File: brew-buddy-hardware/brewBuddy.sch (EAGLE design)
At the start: 3 parts

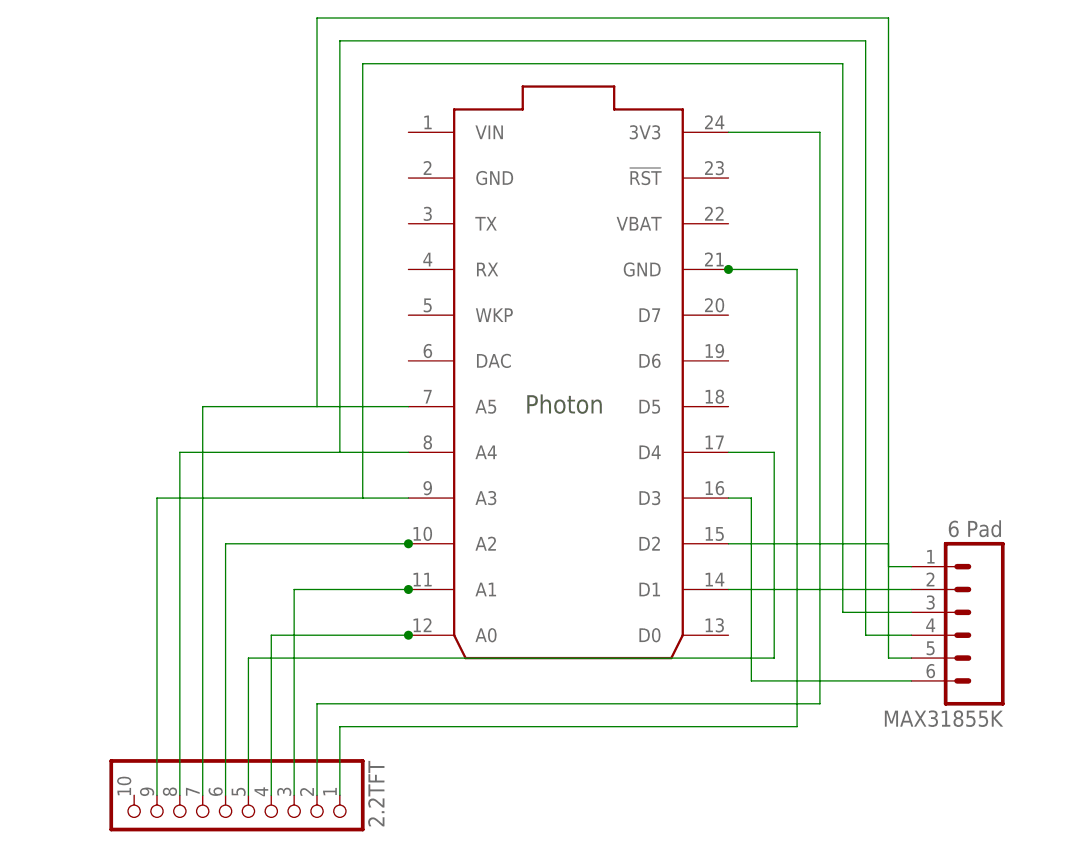
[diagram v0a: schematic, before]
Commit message: updated schematic and board for Argon
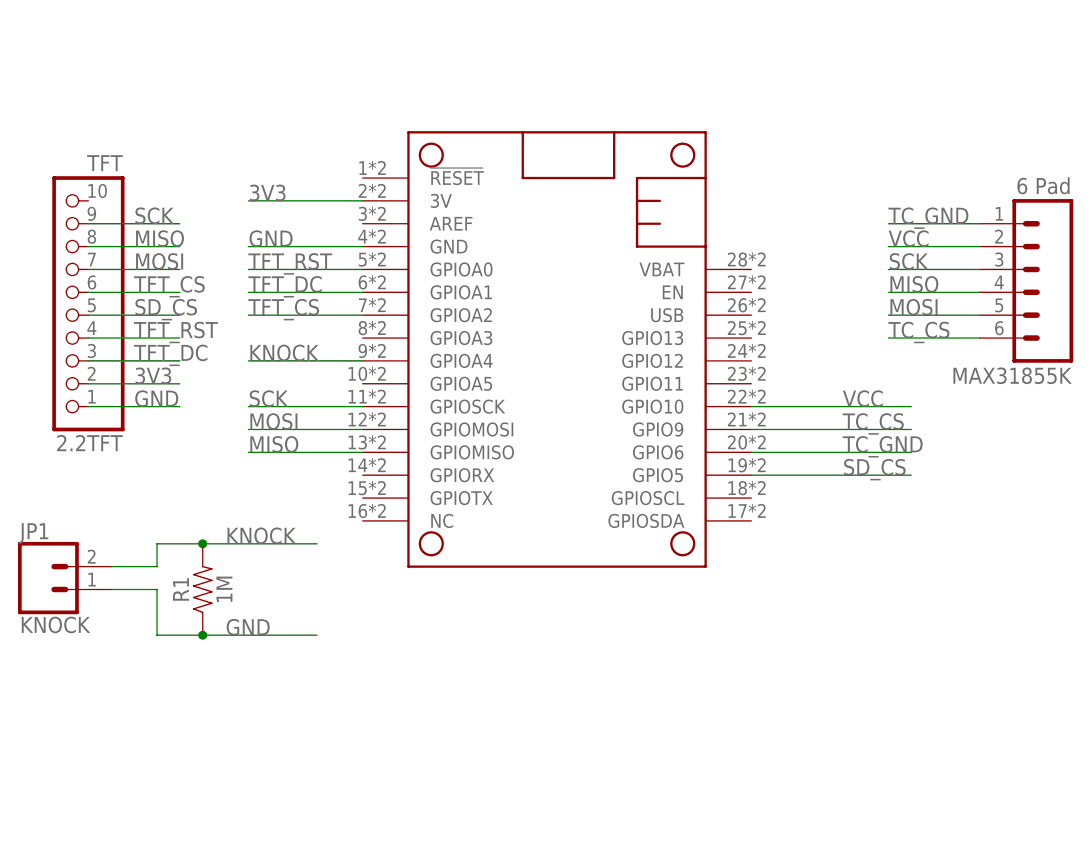
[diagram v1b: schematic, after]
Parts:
- removed U$1: PHOTON_WITH_HEADERS, Spark:PHOTON_WITH_HEADERS
- added JP1: KNOCK, SparkFun-Connectors:CONN_025MM
- added MS1: FEATHERWING_SMTDUAL, Particle-Mesh:FEATHERWING_SMTDUAL
- added R1: 1M, SparkFun-Resistors:RESISTOR0805
- 2.2TFT: value (none) -> TFT
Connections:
- removed net N$1: MAX31855K.1, U$1.D2
- removed net N$10: 2.2TFT.4, U$1.A0
- removed net N$11: 2.2TFT.3, U$1.A1
- removed net N$12: 2.2TFT.2, U$1.3V3
- removed net N$13: 2.2TFT.1, U$1.GND@21
- removed net N$2: MAX31855K.2, U$1.D1
- removed net N$3: MAX31855K.6, U$1.D3
- removed net N$4: 2.2TFT.9, MAX31855K.3, U$1.A3
- removed net N$5: 2.2TFT.8, MAX31855K.4, U$1.A4
- removed net N$6: 2.2TFT.7, MAX31855K.5, U$1.A5
- removed net N$7: 2.2TFT.5, U$1.D4
- removed net N$9: 2.2TFT.6, U$1.A2
- new net 3V3: 2.2TFT.2, MS1.3V
- new net GND: 2.2TFT.1, JP1.1, MS1.GND, R1.1
- new net KNOCK: JP1.2, MS1.GPIOA4, R1.2
- new net MISO: 2.2TFT.8, MAX31855K.4, MS1.GPIOMISO
- new net MOSI: 2.2TFT.7, MAX31855K.5, MS1.GPIOMOSI
- new net SCK: 2.2TFT.9, MAX31855K.3, MS1.GPIOSCK
- new net SD_CS: 2.2TFT.5, MS1.GPIO5
- new net TC_CS: MAX31855K.6, MS1.GPIO9
- new net TC_GND: MAX31855K.1, MS1.GPIO6
- new net TFT_CS: 2.2TFT.6, MS1.GPIOA2
- new net TFT_DC: 2.2TFT.3, MS1.GPIOA1
- new net TFT_RST: 2.2TFT.4, MS1.GPIOA0
- new net VCC: MAX31855K.2, MS1.GPIO10
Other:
- moved on the sheet: 2.2TFT, MAX31855K
